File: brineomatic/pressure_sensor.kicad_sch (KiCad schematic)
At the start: 8 parts, among them J12 SENSOR

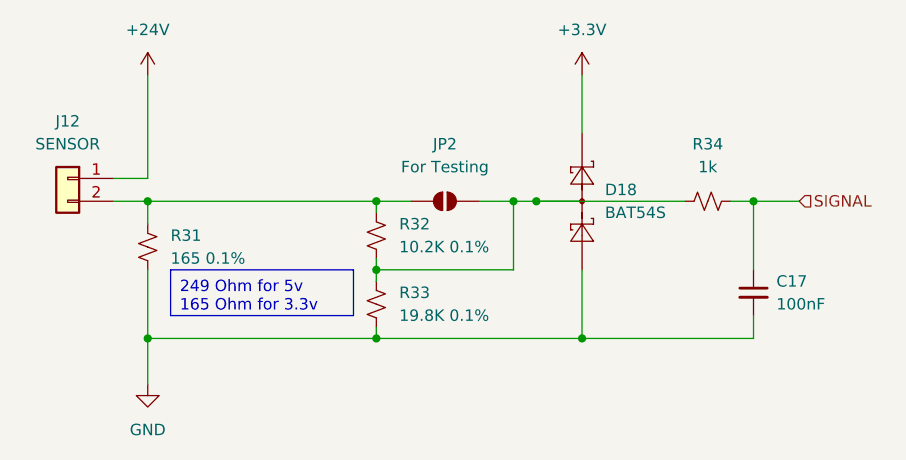
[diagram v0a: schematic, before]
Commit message: starting to look good.
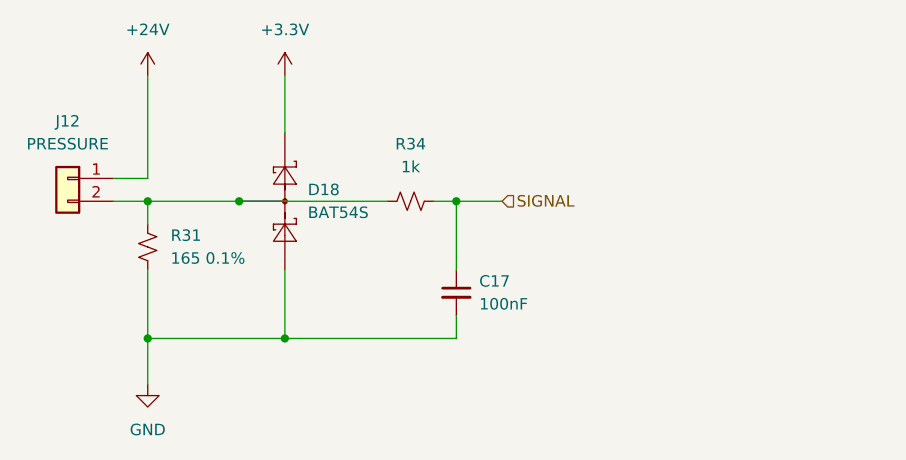
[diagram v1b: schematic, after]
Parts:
- removed JP2: For Testing, Jumper:SolderJumper-2_P1.3mm_Open_RoundedPad1.0x1.5mm, symbol Jumper:SolderJumper_2_Open
- removed R32: 10.2K 0.1%, Resistor_SMD:R_1206_3216Metric_Pad1.30x1.75mm_HandSolder, symbol Device:R_Small_US
- removed R33: 19.8K 0.1%, Resistor_SMD:R_1206_3216Metric_Pad1.30x1.75mm_HandSolder, symbol Device:R_Small_US
- J12: value SENSOR -> PRESSURE; footprint TerminalBlock_Phoenix:TerminalBlock_Phoenix_PT-1,5-2-3.5-H_1x02_P3.50mm_Horizontal -> Connector_JST:JST_PH_S2B-PH-K_1x02_P2.00mm_Horizontal
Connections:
- net at J12.2 (Pin_2), R31.2: now also D18.3 (COM), R34.1
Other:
- moved on the sheet: C17, D18, R34
